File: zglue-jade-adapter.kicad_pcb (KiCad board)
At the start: 8 copper layers, 25 x 20 mm, 63 parts, among them J1 543630489, J2 543630489, U1 zGlue-Jade

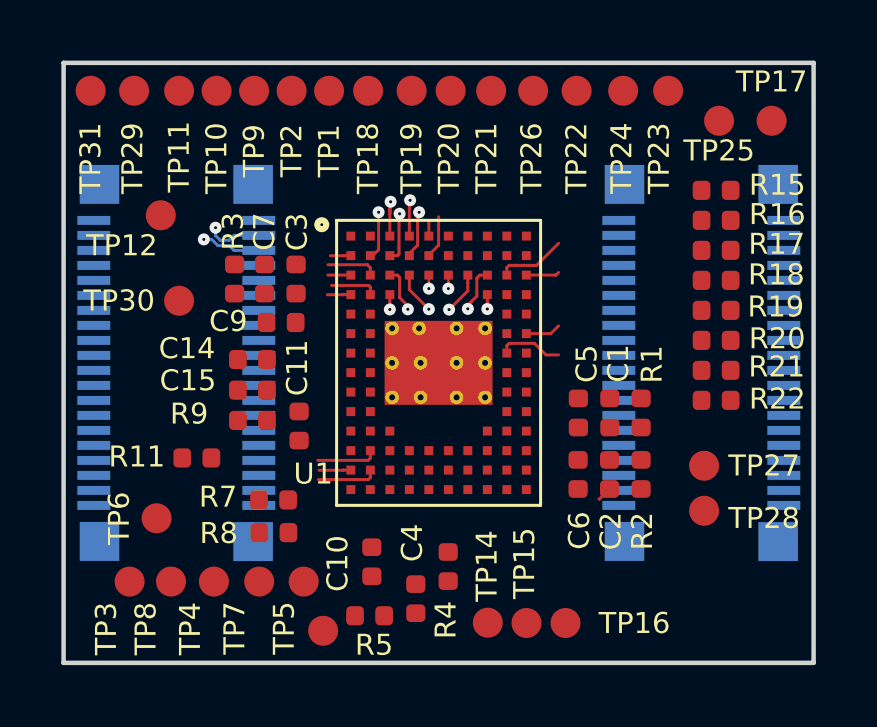
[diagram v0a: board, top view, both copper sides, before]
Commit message: Add initial layout
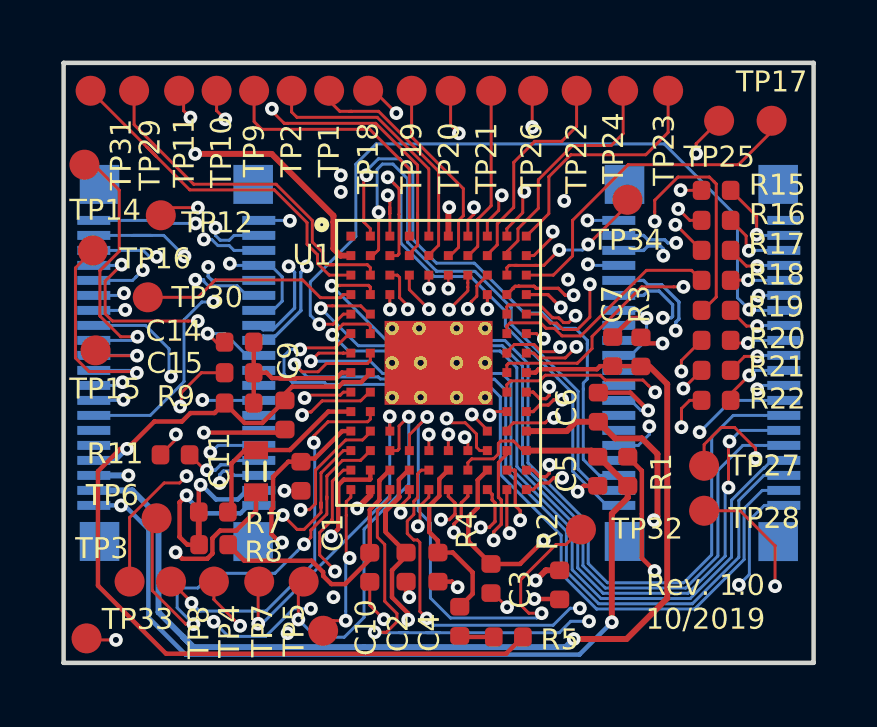
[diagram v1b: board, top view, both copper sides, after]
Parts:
- added TP32: TP_SMD1MM, antmicro-footprints:Testpoint_smd_1mm, F.Cu at (17.2, 15.6)
- added TP33: TP_SMD1MM, antmicro-footprints:Testpoint_smd_1mm, F.Cu at (0.76, 19.2)
- added TP34: TP_SMD1MM, antmicro-footprints:Testpoint_smd_1mm, F.Cu at (18.8, 4.62)
- C11: value C_100n_0402_6V3 -> C_1u_0603; footprint antmicro-footprints:0402-cap -> antmicro-footprints:0603-cap
- moved TP14 20.3 mm to (0.69, 3.45), turned to 0 degrees
- moved TP16 20.0 mm to (0.97, 6.31), turned to 0 degrees
- moved TP15 16.9 mm to (1.06, 9.64), turned to 0 degrees
- moved R3 13.8 mm to (19.2, 9.64)
- moved C3 11.9 mm to (14.2, 17.2), turned to 270 degrees
- moved C7 11.9 mm to (18.3, 9.63)
- moved C1 10.5 mm to (7.91, 13.8), turned to 270 degrees
- moved C2 7.45 mm to (11.4, 16.8)
- moved R5 4.68 mm to (14.8, 19.1), turned to 0 degrees
- moved R2 4.57 mm to (16.5, 17.4), turned to 90 degrees
- moved C9 3.08 mm to (7.37, 11.7), turned to 270 degrees
- moved C6 2.34 mm to (17.8, 11.5), turned to 90 degrees
- moved C11 2.08 mm to (6.41, 13.6)
- moved C5 2.05 mm to (17.8, 13.6), turned to 270 degrees
- moved R7 2.05 mm to (4.99, 15.0)
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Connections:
- C1 pad 1: /3V3_SYS -> /3V3
- C2 pad 1: /1V8_SYS -> /1V8
- C3 pad 1: /2V5_SYS -> /2V5
- C4 pad 1: /1V2_SYS -> /1V2
- R4 pad 2: /1V2_SYS -> Net-(R4-Pad2)
- R5 pad 1: /1V2_SYS -> Net-(R4-Pad2)
- U1 pad L10: /3V3_SYS -> /1V8_SYS
- U1 pad M10: /1V8_SYS -> /3V3_SYS
- U1 pad N1: /VDDIO_BST -> /BOOST_OUT
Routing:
- net /3V3_SYS: track 0.69 -> 54.2 mm, vias 0 -> 3
- net GND: track 2.51 -> 52.1 mm, vias 0 -> 27
- net /2V5_SYS: track 0.00 -> 36.8 mm, vias 0 -> 1
- net /1V8_SYS: track 0.00 -> 34.7 mm, vias 0 -> 3
- net /I2C_0_SDA: track 0.00 -> 31.6 mm, vias 0 -> 2
- net /I2C_0_SCL: track 0.00 -> 31.5 mm, vias 0 -> 2
- net /1V2_SYS: track 0.00 -> 31.3 mm, vias 0 -> 1
- net /USB_D_P: track 0.00 -> 31.1 mm, vias 0 -> 3
- net /USB_D_N: track 0.00 -> 30.7 mm, vias 0 -> 3
- net /PIO16: track 2.17 -> 32.2 mm, vias 0 -> 3
- net /USB_DET: track 0.00 -> 29.7 mm, vias 0 -> 4
- net /DONE: track 1.38 -> 29.6 mm, vias 1 -> 3
- net /FLASH_IO3: track 0.00 -> 28.2 mm, vias 0 -> 1
- net /FLASH_IO2: track 0.00 -> 27.6 mm, vias 0 -> 1
- net /FLASH_IO0: track 0.00 -> 27.4 mm, vias 0 -> 1
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- added copper zone on Ground_Layer2, net GND
- added copper zone on Ground_layer1, net GND
- removed copper zone on Power_Layer2, net /1V2_SYS
- removed copper zone on Power_Layer1, net /3V3_SYS
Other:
- copper layers 8 -> 6
- net class Default: via_dia 0.4 -> 0.457; via_drill 0.1 -> 0.2
- rule via_min_size: 0.4 -> 0.457
- board text added: "Rev. 1.0 10/2019"

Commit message: Tune differential pairs
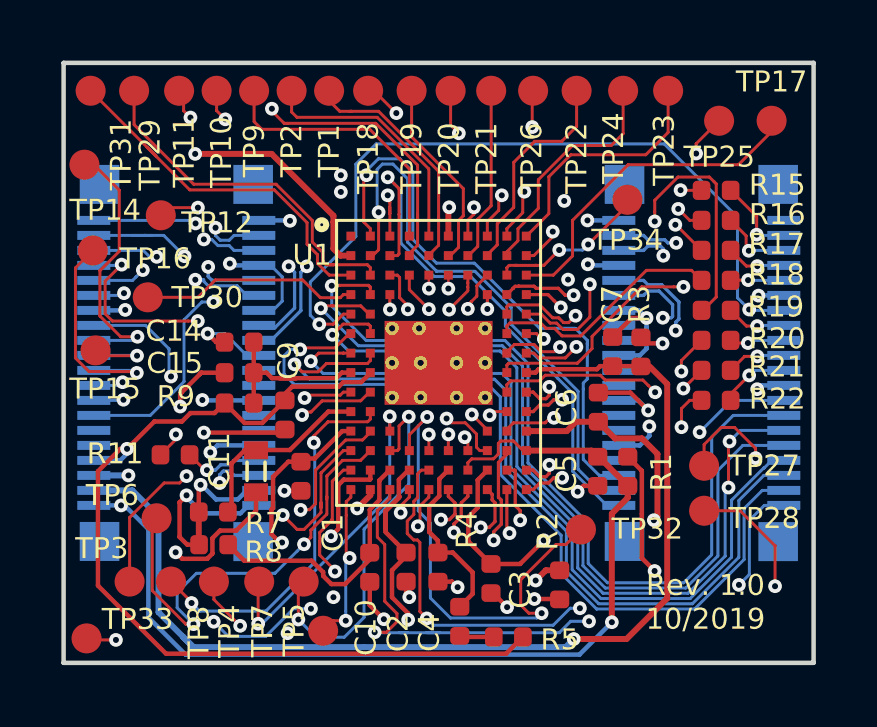
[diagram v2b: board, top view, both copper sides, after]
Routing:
- net /CSI_D2_IN_N: track 18.8 -> 23.4 mm
- net /CSI_CLK_IN_N: track 19.1 -> 23.4 mm
- net /CSI_CLK_IN_P: track 19.6 -> 23.4 mm
- net /CSI_D2_IN_P: track 20.5 -> 23.3 mm
- net /CSI_D1_IN_P: track 21.1 -> 23.4 mm
- net GND: track 52.1 -> 53.2 mm
- net /CSI_D1_OUT_P: track 12.5 -> 13.4 mm
- net /CSI_D1_OUT_N: track 12.8 -> 13.8 mm
- net /USB_D_P: track 31.1 -> 31.9 mm
- net /CSI_CLK_OUT_N: track 13.2 -> 13.9 mm
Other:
- board text added: "0.02mm"
- board text added: "0.035mm"
- board text added: "0.12"
- board text added: "0.12mm"
- board text added: "0.14"
- board text added: "0.2"
- board text added: "1"
- board text added: "3.5"
- board text added: "4.2"
- board text added: "Bottom Layer"
- board text added: "Bottom Solder"
- board text added: "Constant"
- board text added: "Copper"
- board text added: "Core 1"
- board text added: "Core 2"
- board text added: "Dielectric 1"
- board text added: "Dielectric 3"
- board text added: "Dielectric2"
- board text added: "FR-4"
- board text added: "Ground Plane 1"
- board text added: "Ground Plane 2"
- board text added: "Layer"
- board text added: "Material"
- board text added: "Name"
- board text added: "Signal Layer 1"
- board text added: "Signal Layer 2"
- board text added: "Solder Resist"
- board text added: "Thickness"
- board text added: "Top Layer"
- board text added: "Top Solder"
